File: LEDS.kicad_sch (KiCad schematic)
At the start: 12 parts

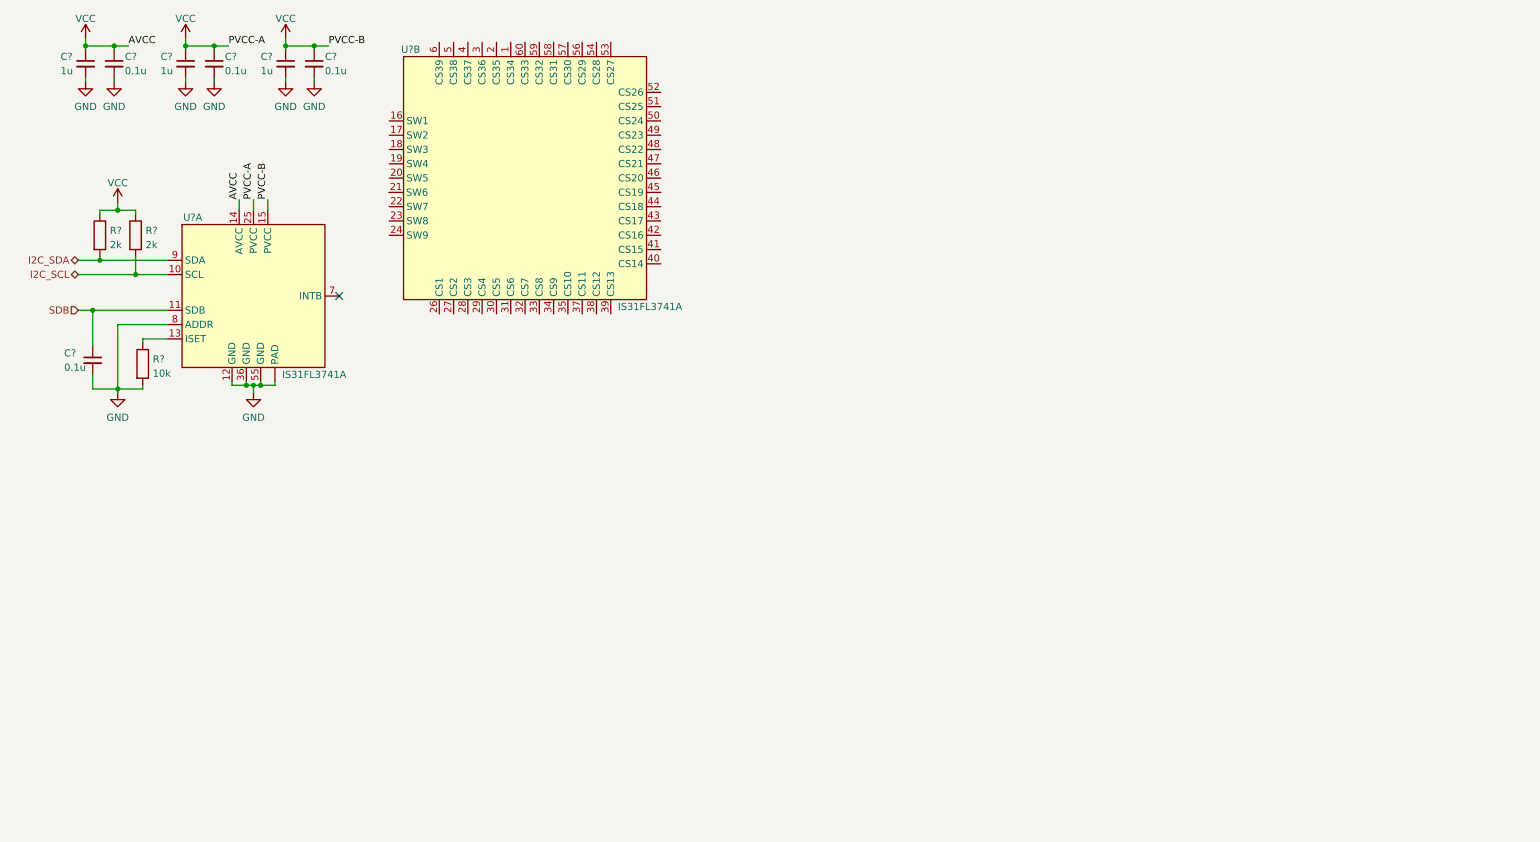
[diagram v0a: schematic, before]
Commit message: first draft
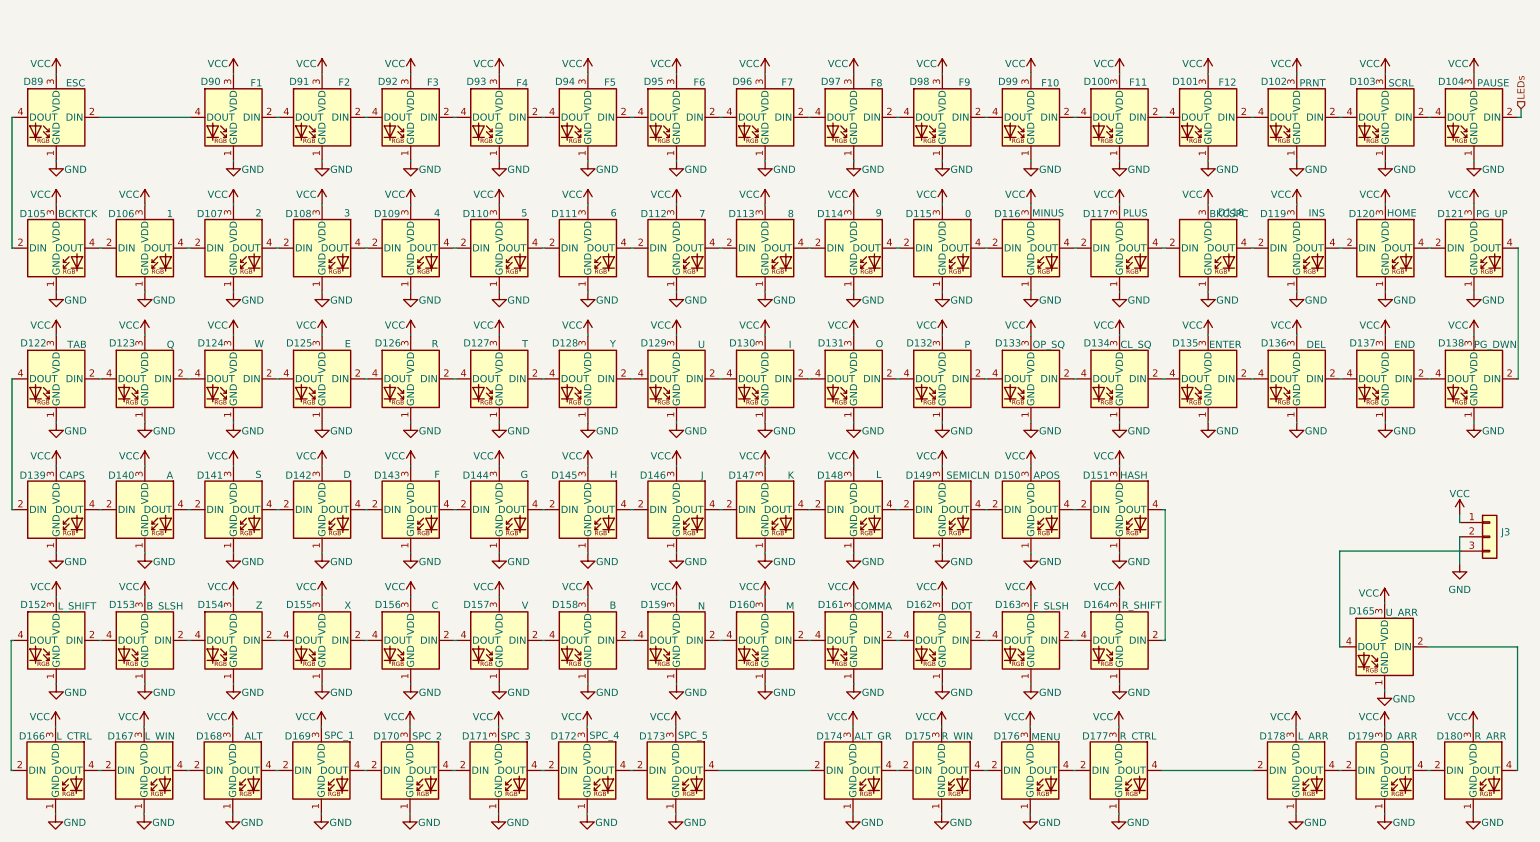
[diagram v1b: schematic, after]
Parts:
- removed C? (x4): 0.1u, symbol Device:C_Small
- removed C? (x3): 1u, symbol Device:C_Small
- removed R?: 10k, symbol Device:R
- removed R? (x2): 2k, symbol Device:R
- removed U? (x2): IS31FL3741A, symbol Custom:IS31FL3741A
- added D100, D101, D102, D103, D104, D105, D106, D107, D108, D109, D110, D111, D112, D113, D114, D115, D116, D117, D118, D119, D120, D121, D122, D123, D124, D125, D126, D127, D128, D129, D130, D131, D132, D133, D134, D135, D136, D137, D138, D139, D140, D141, D142, D143, D144, D145, D146, D147, D148, D149, D150, D151, D152, D153, D154, D155, D156, D157, D158, D159, D160, D161, D162, D163, D164, D165, D166, D167, D168, D169, D170, D171, D172, D173, D174, D175, D176, D177, D178, D179, D180, D89, D90, D91, D92, D93, D94, D95, D96, D97, D98, D99: SK6803MINI-E, symbol Custom:SK6803MINI-E
- added J3: Conn_01x03, symbol Connector_Generic:Conn_01x03
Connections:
- net GND: now also D100.1 (GND), D101.1 (GND), D102.1 (GND), D103.1 (GND), D104.1 (GND), D105.1 (GND), D106.1 (GND), D107.1 (GND), D108.1 (GND), D109.1 (GND), D110.1 (GND), D111.1 (GND), D112.1 (GND), D113.1 (GND), D114.1 (GND), D115.1 (GND), D116.1 (GND), D117.1 (GND), D118.1 (GND), D119.1 (GND), D120.1 (GND), D121.1 (GND), D122.1 (GND), D123.1 (GND), D124.1 (GND), D125.1 (GND), D126.1 (GND), D127.1 (GND), D128.1 (GND), D129.1 (GND), D130.1 (GND), D131.1 (GND), D132.1 (GND), D133.1 (GND), D134.1 (GND), D135.1 (GND), D136.1 (GND), D137.1 (GND), D138.1 (GND), D139.1 (GND), D140.1 (GND), D141.1 (GND), D142.1 (GND), D143.1 (GND), D144.1 (GND), D145.1 (GND), D146.1 (GND), D147.1 (GND), D148.1 (GND), D149.1 (GND), D150.1 (GND), D151.1 (GND), D152.1 (GND), D153.1 (GND), D154.1 (GND), D155.1 (GND), D156.1 (GND), D157.1 (GND), D158.1 (GND), D159.1 (GND), D160.1 (GND), D161.1 (GND), D162.1 (GND), D163.1 (GND), D164.1 (GND), D165.1 (GND), D166.1 (GND), D167.1 (GND), D168.1 (GND), D169.1 (GND), D170.1 (GND), D171.1 (GND), D172.1 (GND), D173.1 (GND), D174.1 (GND), D175.1 (GND), D176.1 (GND), D177.1 (GND), D178.1 (GND), D179.1 (GND), D180.1 (GND), D89.1 (GND), D90.1 (GND), D91.1 (GND), D92.1 (GND), D93.1 (GND), D94.1 (GND), D95.1 (GND), D96.1 (GND), D97.1 (GND), D98.1 (GND), D99.1 (GND), J3.2 (Pin_2)
- net VCC: now also D100.3 (VDD), D101.3 (VDD), D102.3 (VDD), D103.3 (VDD), D104.3 (VDD), D105.3 (VDD), D106.3 (VDD), D107.3 (VDD), D108.3 (VDD), D109.3 (VDD), D110.3 (VDD), D111.3 (VDD), D112.3 (VDD), D113.3 (VDD), D114.3 (VDD), D115.3 (VDD), D116.3 (VDD), D117.3 (VDD), D118.3 (VDD), D119.3 (VDD), D120.3 (VDD), D121.3 (VDD), D122.3 (VDD), D123.3 (VDD), D124.3 (VDD), D125.3 (VDD), D126.3 (VDD), D127.3 (VDD), D128.3 (VDD), D129.3 (VDD), D130.3 (VDD), D131.3 (VDD), D132.3 (VDD), D133.3 (VDD), D134.3 (VDD), D135.3 (VDD), D136.3 (VDD), D137.3 (VDD), D138.3 (VDD), D139.3 (VDD), D140.3 (VDD), D141.3 (VDD), D142.3 (VDD), D143.3 (VDD), D144.3 (VDD), D145.3 (VDD), D146.3 (VDD), D147.3 (VDD), D148.3 (VDD), D149.3 (VDD), D150.3 (VDD), D151.3 (VDD), D152.3 (VDD), D153.3 (VDD), D154.3 (VDD), D155.3 (VDD), D156.3 (VDD), D157.3 (VDD), D158.3 (VDD), D159.3 (VDD), D160.3 (VDD), D161.3 (VDD), D162.3 (VDD), D163.3 (VDD), D164.3 (VDD), D165.3 (VDD), D166.3 (VDD), D167.3 (VDD), D168.3 (VDD), D169.3 (VDD), D170.3 (VDD), D171.3 (VDD), D172.3 (VDD), D173.3 (VDD), D174.3 (VDD), D175.3 (VDD), D176.3 (VDD), D177.3 (VDD), D178.3 (VDD), D179.3 (VDD), D180.3 (VDD), D89.3 (VDD), D90.3 (VDD), D91.3 (VDD), D92.3 (VDD), D93.3 (VDD), D94.3 (VDD), D95.3 (VDD), D96.3 (VDD), D97.3 (VDD), D98.3 (VDD), D99.3 (VDD), J3.1 (Pin_1)
- new net: D141.4 (DOUT), D142.2 (DIN)
- new net: D142.4 (DOUT), D143.2 (DIN)
- new net: D148.4 (DOUT), D149.2 (DIN)
- new net: D149.4 (DOUT), D150.2 (DIN)
- new net: D134.2 (DIN), D135.4 (DOUT)
- new net: D133.2 (DIN), D134.4 (DOUT)
- new net: D105.4 (DOUT), D106.2 (DIN)
- new net: D106.4 (DOUT), D107.2 (DIN)
- new net: D130.2 (DIN), D131.4 (DOUT)
- new net: D129.2 (DIN), D130.4 (DOUT)
- new net: D100.2 (DIN), D101.4 (DOUT)
- new net: D100.4 (DOUT), D99.2 (DIN)
- new net: D126.2 (DIN), D127.4 (DOUT)
- new net: D125.2 (DIN), D126.4 (DOUT)
- new net: D165.2 (DIN), D180.4 (DOUT)
- new net: D165.4 (DOUT), J3.3 (Pin_3)
- new net: D97.2 (DIN), D98.4 (DOUT)
- new net: D96.2 (DIN), D97.4 (DOUT)
- new net: D109.4 (DOUT), D110.2 (DIN)
- new net: D110.4 (DOUT), D111.2 (DIN)
- new net: D147.4 (DOUT), D148.2 (DIN)
- new net: D146.4 (DOUT), D147.2 (DIN)
- new net: D123.2 (DIN), D124.4 (DOUT)
- new net: D122.2 (DIN), D123.4 (DOUT)
- new net: D122.4 (DOUT), D139.2 (DIN)
- new net: D171.4 (DOUT), D172.2 (DIN)
- new net: D172.4 (DOUT), D173.2 (DIN)
- new net: D94.2 (DIN), D95.4 (DOUT)
- new net: D93.2 (DIN), D94.4 (DOUT)
- new net: D101.2 (DIN), D102.4 (DOUT)
- new net: D105.2 (DIN), D89.4 (DOUT)
- new net: D90.2 (DIN), D91.4 (DOUT)
- new net: D89.2 (DIN), D90.4 (DOUT)
- new net: D95.2 (DIN), D96.4 (DOUT)
- new net: D174.4 (DOUT), D175.2 (DIN)
- new net: D175.4 (DOUT), D176.2 (DIN)
- new net: D116.4 (DOUT), D117.2 (DIN)
- new net: D117.4 (DOUT), D118.2 (DIN)
- new net: D161.2 (DIN), D162.4 (DOUT)
- new net: D160.2 (DIN), D161.4 (DOUT)
- new net: D145.4 (DOUT), D146.2 (DIN)
- new net: D158.2 (DIN), D159.4 (DOUT)
- new net: D157.2 (DIN), D158.4 (DOUT)
- new net: D170.4 (DOUT), D171.2 (DIN)
- new net: D121.4 (DOUT), D138.2 (DIN)
- new net: D137.2 (DIN), D138.4 (DOUT)
- new net: D118.4 (DOUT), D119.2 (DIN)
- new net: D124.2 (DIN), D125.4 (DOUT)
- new net: D152.4 (DOUT), D166.2 (DIN)
- new net: D166.4 (DOUT), D167.2 (DIN)
- new net: D169.4 (DOUT), D170.2 (DIN)
- new net: D152.2 (DIN), D153.4 (DOUT)
- new net: D173.4 (DOUT), D174.2 (DIN)
- new net: D102.2 (DIN), D103.4 (DOUT)
- new net: D92.2 (DIN), D93.4 (DOUT)
- new net: D140.4 (DOUT), D141.2 (DIN)
- new net: D132.2 (DIN), D133.4 (DOUT)
- new net: D131.2 (DIN), D132.4 (DOUT)
- new net: D167.4 (DOUT), D168.2 (DIN)
- new net: D168.4 (DOUT), D169.2 (DIN)
- new net: D153.2 (DIN), D154.4 (DOUT)
- new net: D135.2 (DIN), D136.4 (DOUT)
- new net: D150.4 (DOUT), D151.2 (DIN)
- new net: D139.4 (DOUT), D140.2 (DIN)
- new net: D103.2 (DIN), D104.4 (DOUT)
- new net: D159.2 (DIN), D160.4 (DOUT)
- new net: D154.2 (DIN), D155.4 (DOUT)
- new net: D143.4 (DOUT), D144.2 (DIN)
- new net: D112.4 (DOUT), D113.2 (DIN)
- new net: D113.4 (DOUT), D114.2 (DIN)
- new net: D176.4 (DOUT), D177.2 (DIN)
- new net: D120.4 (DOUT), D121.2 (DIN)
- new net: D111.4 (DOUT), D112.2 (DIN)
- new net: D108.4 (DOUT), D109.2 (DIN)
- new net: D128.2 (DIN), D129.4 (DOUT)
- new net: D107.4 (DOUT), D108.2 (DIN)
- new net: D162.2 (DIN), D163.4 (DOUT)
- new net: D119.4 (DOUT), D120.2 (DIN)
- new net: D177.4 (DOUT), D178.2 (DIN)
- new net: D178.4 (DOUT), D179.2 (DIN)
- new net: D115.4 (DOUT), D116.2 (DIN)
- new net: D114.4 (DOUT), D115.2 (DIN)
- new net: D156.2 (DIN), D157.4 (DOUT)
- new net: D127.2 (DIN), D128.4 (DOUT)
- new net: D151.4 (DOUT), D164.2 (DIN)
- new net: D144.4 (DOUT), D145.2 (DIN)
- new net: D91.2 (DIN), D92.4 (DOUT)
- new net: D155.2 (DIN), D156.4 (DOUT)
- new net: D98.2 (DIN), D99.4 (DOUT)
- new net: D136.2 (DIN), D137.4 (DOUT)
- new net: D163.2 (DIN), D164.4 (DOUT)
- new net: D179.4 (DOUT), D180.2 (DIN)
- new net LEDs: D104.2 (DIN)
- no-connect marks 1 -> 0
